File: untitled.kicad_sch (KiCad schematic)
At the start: 37 parts, among them J13 RaspPi_Conn, J15 UART_Bridge_TXRX, J16 Test_Conns, J3 USB_B_Micro, SW1 SW_Push, SW2 SW_Push, U3 ESP32-S3-WROOM-1

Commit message: after connor fixed footprints and billy started layout
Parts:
- C1, C11, C2: footprint CustomComponents:CAPC2012X95N_ -> LocalComponents:CAPC2012X95N_
- C8: footprint CustomComponents:CAPC1608X100N -> LocalComponents:CAPC1608X100N
- C9: footprint CustomComponents:CAPC1005X55N -> LocalComponents:CAPC1005X55N
- D11, D16: footprint CustomComponents:ESD5V0LBTP -> LocalComponents:ESD5V0LBTP
- J3: footprint CustomComponents:CONN_UB-MC5BR3-SDWP604-4S-TF_JST -> LocalComponents:CONN_UB-MC5BR3-SDWP604-4S-TF_JST
- R13, R21: footprint CustomComponents:RESC1005X40 -> LocalComponents:RESC1005X40
- R14: footprint CustomComponents:STA_RMCF0402_STP -> LocalComponents:STA_RMCF0402_STP
- R35: footprint CustomComponents:RESC2012X60N -> LocalComponents:RESC2012X60N
- SW1, SW2: footprint (none) -> LocalComponents:ESB335_PAN
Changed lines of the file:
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@@
 			)
 		)
-		(property "Footprint" "CustomComponents:CAPC2012X95N_"
+		(property "Footprint" "LocalComponents:CAPC2012X95N_"
 			(at 113.03 101.2952 0)
 			(effects
@@
 			)
 		)
-		(property "Footprint" "CustomComponents:CAPC2012X95N_"
+		(property "Footprint" "LocalComponents:CAPC2012X95N_"
 			(at 35.2552 44.45 0)
 			(effects
@@
 			)
 		)
-		(property "Footprint" "CustomComponents:CAPC1005X55N"
+		(property "Footprint" "LocalComponents:CAPC1005X55N"
 			(at 158.4452 40.64 0)
 			(effects
@@
 			)
 		)
-		(property "Footprint" "CustomComponents:ESD5V0LBTP"
+		(property "Footprint" "LocalComponents:ESD5V0LBTP"
 			(at 55.88 113.03 0)
 			(effects
@@
 			)
 		)
-		(property "Footprint" "CustomComponents:RESC1005X40"
+		(property "Footprint" "LocalComponents:RESC1005X40"
 			(at 28.702 77.47 90)
 			(effects
@@
 			)
 		)
-		(property "Footprint" "CustomComponents:RESC1005X40"
+		(property "Footprint" "LocalComponents:RESC1005X40"
 			(at 37.592 77.47 90)
 			(effects
@@
 			)
 		)
-		(property "Footprint" ""
+		(property "Footprint" "LocalComponents:ESB335_PAN"
 			(at 109.22 88.9 0)
 			(effects
@@
 			)
 		)
-		(property "Datasheet" "~"
+		(property "Datasheet" "https://www.digikey.com/en/products/detail/panasonic-electronic-components/ESB-33535A/3873298"
 			(at 109.22 88.9 0)
 			(effects
@@
 			)
 		)
-		(property "Footprint" "CustomComponents:STA_RMCF0402_STP"
+		(property "Footprint" "LocalComponents:STA_RMCF0402_STP"
 			(at 155.702 25.4 90)
 			(effects
@@
 			)
 		)
-		(property "Footprint" "CustomComponents:RESC2012X60N"
+		(property "Footprint" "LocalComponents:RESC2012X60N"
 			(at 14.732 115.57 90)
 			(effects
@@
 			)
 		)
-		(property "Footprint" ""
+		(property "Footprint" "LocalComponents:ESB335_PAN"
 			(at 109.22 125.73 0)
 			(effects
@@
 			)
 		)
-		(property "Datasheet" "~"
+		(property "Datasheet" "https://www.digikey.com/en/products/detail/panasonic-electronic-components/ESB-33535A/3873298"
 			(at 109.22 125.73 0)
 			(effects
@@
 			)
 		)
-		(property "Footprint" "CustomComponents:CONN_UB-MC5BR3-SDWP604-4S-TF_JST"
+		(property "Footprint" "LocalComponents:CONN_UB-MC5BR3-SDWP604-4S-TF_JST"
 			(at 22.86 102.87 0)
 			(effects
@@
 			)
 		)
-		(property "Footprint" "CustomComponents:CAPC2012X95N_"
+		(property "Footprint" "LocalComponents:CAPC2012X95N_"
 			(at 113.03 138.1252 0)
 			(effects
@@
 			)
 		)
-		(property "Footprint" "CustomComponents:CAPC1608X100N"
+		(property "Footprint" "LocalComponents:CAPC1608X100N"
 			(at 23.8252 44.45 0)
 			(effects
@@
 			)
 		)
-		(property "Footprint" "CustomComponents:ESD5V0LBTP"
+		(property "Footprint" "LocalComponents:ESD5V0LBTP"
 			(at 46.99 118.11 0)
 			(effects

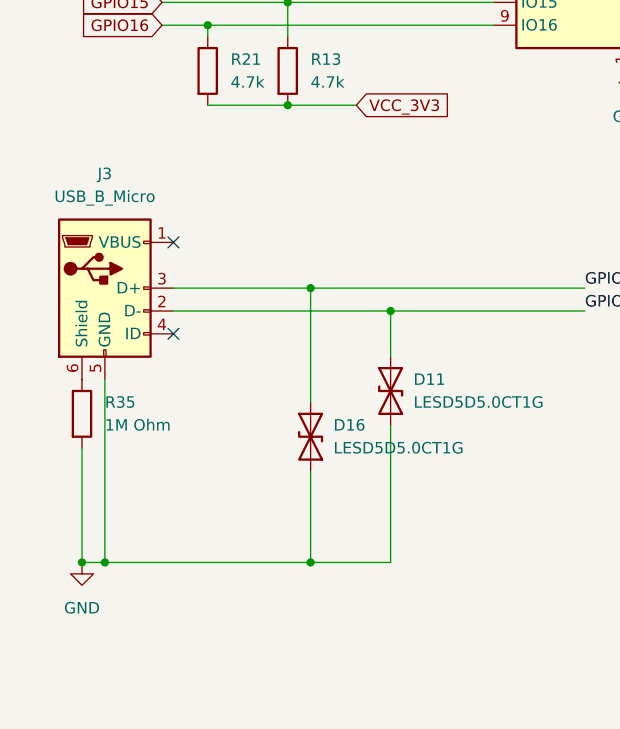
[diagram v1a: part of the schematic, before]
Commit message: pcb layout done, billy watching over us
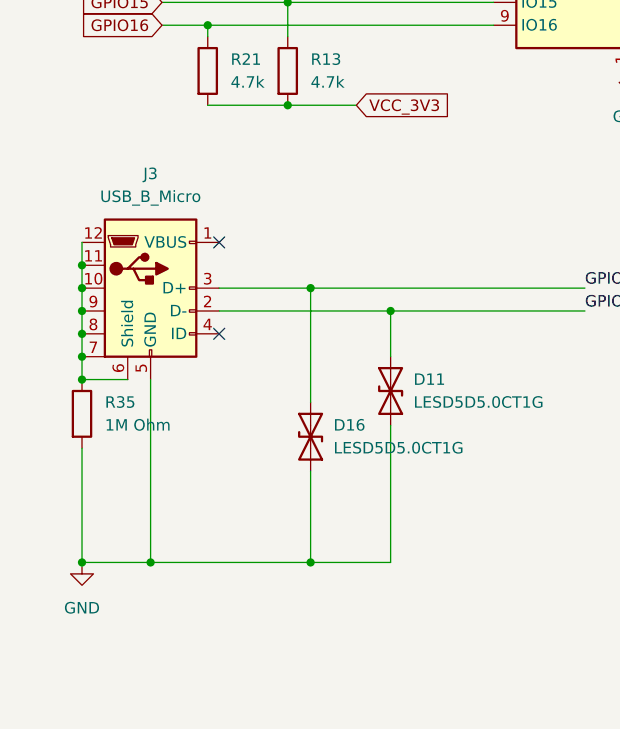
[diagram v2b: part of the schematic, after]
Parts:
- SW1, SW2: footprint LocalComponents:ESB335_PAN -> Button_Switch_THT:SW_PUSH-12mm
- TP1, TP2: footprint (none) -> TestPoint:TestPoint_Pad_D1.5mm
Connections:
- net at J3.6 (Shield), R35.1: now also J3.10, J3.11, J3.12, J3.7, J3.8, J3.9
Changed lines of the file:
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@@
 	)
 	(junction
+		(at 16.51 99.06)
+		(diameter 0)
+		(color 0 0 0 0)
+	)
+	(junction
+		(at 16.51 101.6)
+		(diameter 0)
+		(color 0 0 0 0)
+	)
+	(junction
 		(at 220.98 73.66)
 		(diameter 0)
@@
 	)
 	(junction
+		(at 16.51 106.68)
+		(diameter 0)
+		(color 0 0 0 0)
+	)
+	(junction
 		(at 165.1 120.65)
 		(diameter 0)
@@
 	)
 	(junction
-		(at 19.05 132.08)
+		(at 116.84 100.33)
 		(diameter 0)
 		(color 0 0 0 0)
 	)
 	(junction
-		(at 116.84 100.33)
+		(at 50.8 104.14)
 		(diameter 0)
 		(color 0 0 0 0)
 	)
 	(junction
-		(at 50.8 104.14)
+		(at 24.13 132.08)
 		(diameter 0)
 		(color 0 0 0 0)
@@
 	)
 	(junction
+		(at 16.51 109.22)
+		(diameter 0)
+		(color 0 0 0 0)
+	)
+	(junction
 		(at 127 25.4)
 		(diameter 0)
@@
 	)
 	(junction
+		(at 16.51 111.76)
+		(diameter 0)
+		(color 0 0 0 0)
+	)
+	(junction
 		(at 39.37 69.85)
 		(diameter 0)
@@
 	)
 	(junction
+		(at 16.51 104.14)
+		(diameter 0)
+		(color 0 0 0 0)
+	)
+	(junction
 		(at 226.06 86.36)
 		(diameter 0)
@@
 	)
 	(no_connect
-		(at 26.67 96.52)
+		(at 31.75 96.52)
 	)
 	(no_connect
@@
 	)
 	(no_connect
-		(at 26.67 106.68)
+		(at 31.75 106.68)
 	)
 	(no_connect
@@
 	(wire
 		(pts
+			(xy 16.51 99.06) (xy 16.51 101.6)
+		)
+		(stroke
+			(width 0)
+			(type default)
+		)
+	)
+	(wire
+		(pts
 			(xy 226.06 73.66) (xy 220.98 73.66)
 		)
@@
 	(wire
 		(pts
-			(xy 92.71 62.23) (xy 95.25 62.23)
+			(xy 24.13 132.08) (xy 41.91 132.08)
 		)
 		(stroke
@@
 	(wire
 		(pts
-			(xy 157.48 30.48) (xy 171.45 30.48)
+			(xy 92.71 62.23) (xy 95.25 62.23)
 		)
 		(stroke
@@
 	(wire
 		(pts
-			(xy 19.05 132.08) (xy 41.91 132.08)
+			(xy 157.48 30.48) (xy 171.45 30.48)
 		)
 		(stroke
@@
 	(wire
 		(pts
+			(xy 16.51 109.22) (xy 16.51 111.76)
+		)
+		(stroke
+			(width 0)
+			(type default)
+		)
+	)
+	(wire
+		(pts
 			(xy 238.76 41.91) (xy 260.35 41.91)
 		)
@@
 	(wire
 		(pts
+			(xy 16.51 101.6) (xy 16.51 104.14)
+		)
+		(stroke
+			(width 0)
+			(type default)
+		)
+	)
+	(wire
+		(pts
 			(xy 165.1 99.06) (xy 165.1 91.44)
 		)
@@
 	(wire
 		(pts
-			(xy 26.67 104.14) (xy 50.8 104.14)
+			(xy 31.75 104.14) (xy 50.8 104.14)
 		)
 		(stroke
@@
 	(wire
 		(pts
-			(xy 16.51 132.08) (xy 19.05 132.08)
+			(xy 16.51 132.08) (xy 24.13 132.08)
 		)
 		(stroke
@@
 	(wire
 		(pts
+			(xy 16.51 106.68) (xy 16.51 109.22)
+		)
+		(stroke
+			(width 0)
+			(type default)
+		)
+	)
+	(wire
+		(pts
 			(xy 157.48 19.05) (xy 157.48 21.59)
 		)
@@
 	(wire
 		(pts
-			(xy 26.67 101.6) (xy 41.91 101.6)
+			(xy 31.75 101.6) (xy 41.91 101.6)
 		)
 		(stroke
@@
 	(wire
 		(pts
+			(xy 21.59 111.76) (xy 16.51 111.76)
+		)
+		(stroke
+			(width 0)
+			(type default)
+		)
+	)
+	(wire
+		(pts
 			(xy 276.86 26.67) (xy 276.86 33.02)
 		)
@@
 	(wire
 		(pts
+			(xy 16.51 96.52) (xy 16.51 99.06)
+		)
+		(stroke
+			(width 0)
+			(type default)
+		)
+	)
+	(wire
+		(pts
 			(xy 22.86 44.45) (xy 22.86 46.99)
 		)
@@
 	(wire
 		(pts
+			(xy 16.51 104.14) (xy 16.51 106.68)
+		)
+		(stroke
+			(width 0)
+			(type default)
+		)
+	)
+	(wire
+		(pts
 			(xy 118.11 30.48) (xy 128.27 30.48)
 		)
@@
 	(wire
 		(pts
-			(xy 19.05 111.76) (xy 19.05 132.08)
+			(xy 24.13 111.76) (xy 24.13 132.08)
 		)
 		(stroke
@@
 			)
 		)
-		(property "Footprint" "LocalComponents:ESB335_PAN"
+		(property "Footprint" "Button_Switch_THT:SW_PUSH-12mm"
 			(at 109.22 88.9 0)
 			(effects
@@
 			)
 		)
-		(property "Footprint" "LocalComponents:ESB335_PAN"
+		(property "Footprint" "Button_Switch_THT:SW_PUSH-12mm"
 			(at 109.22 125.73 0)
 			(effects
@@
 	(symbol
 		(lib_id "Connector:USB_B_Micro")
-		(at 19.05 101.6 0)
+		(at 24.13 101.6 0)
 		(unit 1)
 		(exclude_from_sim no)
@@
 		(fields_autoplaced yes)
 		(property "Reference" "J3"
-			(at 19.05 88.9 0)
+			(at 24.13 88.9 0)
 			(effects
 				(font
@@
 		)
 		(property "Value" "USB_B_Micro"
-			(at 19.05 91.44 0)
+			(at 24.13 91.44 0)
 			(effects
 				(font
@@
 		)
 		(property "Footprint" "LocalComponents:CONN_UB-MC5BR3-SDWP604-4S-TF_JST"
-			(at 22.86 102.87 0)
+			(at 27.94 102.87 0)
 			(effects
 				(font
@@
 		)
 		(property "Datasheet" "https://www.jst-mfg.com/product/pdf/eng/eUB-micro-USB1.pdf"
-			(at 22.86 102.87 0)
+			(at 27.94 102.87 0)
 			(effects
 				(font
@@
 		)
 		(property "Description" "USB Micro Type B connector"
-			(at 19.05 101.6 0)
+			(at 24.13 101.6 0)
 			(effects
 				(font
@@
 		(pin "1"
 		)
+		(pin "12"
+		)
+		(pin "11"
+		)
+		(pin "10"
+		)
+		(pin "9"
+		)
+		(pin "8"
+		)
+		(pin "7"
+		)
 		(instances
 			(project "PCB_draft1"
@@
 			)
 		)
-		(property "Footprint" ""
+		(property "Footprint" "TestPoint:TestPoint_Pad_D1.5mm"
 			(at 121.92 128.27 0)
 			(effects
@@
 			)
 		)
-		(property "Footprint" ""
+		(property "Footprint" "TestPoint:TestPoint_Pad_D1.5mm"
 			(at 121.92 91.44 0)
 			(effects

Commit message: pcb draft 2 from billy
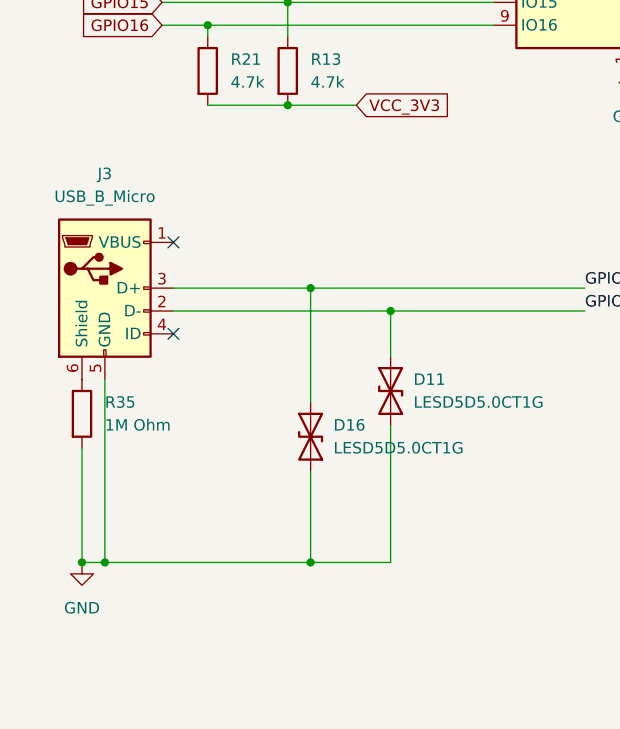
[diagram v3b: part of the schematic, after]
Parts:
- R13, R21: footprint LocalComponents:RESC1005X40 -> Resistor_SMD:R_0805_2012Metric_Pad1.20x1.40mm_HandSolder
- R14: footprint LocalComponents:STA_RMCF0402_STP -> Resistor_SMD:R_0805_2012Metric_Pad1.20x1.40mm_HandSolder
- R35: footprint LocalComponents:RESC2012X60N -> Resistor_SMD:R_0805_2012Metric_Pad1.20x1.40mm_HandSolder
- SW1, SW2: footprint Button_Switch_THT:SW_PUSH-12mm -> LocalComponents:ESB335_PAN
- TP1, TP2: footprint TestPoint:TestPoint_Pad_D1.5mm -> TestPoint_Pad_D1.0mm
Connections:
- new net: J3.6 (Shield), R35.1
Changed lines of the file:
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@@
 	)
 	(junction
-		(at 16.51 99.06)
-		(diameter 0)
-		(color 0 0 0 0)
-	)
-	(junction
-		(at 16.51 101.6)
-		(diameter 0)
-		(color 0 0 0 0)
-	)
-	(junction
 		(at 220.98 73.66)
 		(diameter 0)
@@
 	)
 	(junction
-		(at 16.51 106.68)
-		(diameter 0)
-		(color 0 0 0 0)
-	)
-	(junction
 		(at 165.1 120.65)
 		(diameter 0)
@@
 	)
 	(junction
-		(at 116.84 100.33)
+		(at 19.05 132.08)
 		(diameter 0)
 		(color 0 0 0 0)
 	)
 	(junction
-		(at 50.8 104.14)
+		(at 116.84 100.33)
 		(diameter 0)
 		(color 0 0 0 0)
 	)
 	(junction
-		(at 24.13 132.08)
+		(at 50.8 104.14)
 		(diameter 0)
 		(color 0 0 0 0)
@@
 	)
 	(junction
-		(at 16.51 109.22)
-		(diameter 0)
-		(color 0 0 0 0)
-	)
-	(junction
 		(at 127 25.4)
 		(diameter 0)
@@
 	)
 	(junction
-		(at 16.51 111.76)
-		(diameter 0)
-		(color 0 0 0 0)
-	)
-	(junction
 		(at 39.37 69.85)
 		(diameter 0)
@@
 	)
 	(junction
-		(at 16.51 104.14)
-		(diameter 0)
-		(color 0 0 0 0)
-	)
-	(junction
 		(at 226.06 86.36)
 		(diameter 0)
@@
 	)
 	(no_connect
-		(at 31.75 96.52)
+		(at 26.67 96.52)
 	)
 	(no_connect
@@
 	)
 	(no_connect
-		(at 31.75 106.68)
+		(at 26.67 106.68)
 	)
 	(no_connect
@@
 	(wire
 		(pts
-			(xy 16.51 99.06) (xy 16.51 101.6)
-		)
-		(stroke
-			(width 0)
-			(type default)
-		)
-	)
-	(wire
-		(pts
 			(xy 226.06 73.66) (xy 220.98 73.66)
 		)
@@
 	(wire
 		(pts
-			(xy 24.13 132.08) (xy 41.91 132.08)
+			(xy 92.71 62.23) (xy 95.25 62.23)
 		)
 		(stroke
@@
 	(wire
 		(pts
-			(xy 92.71 62.23) (xy 95.25 62.23)
+			(xy 157.48 30.48) (xy 171.45 30.48)
 		)
 		(stroke
@@
 	(wire
 		(pts
-			(xy 157.48 30.48) (xy 171.45 30.48)
+			(xy 19.05 132.08) (xy 41.91 132.08)
 		)
 		(stroke
@@
 	(wire
 		(pts
-			(xy 16.51 109.22) (xy 16.51 111.76)
-		)
-		(stroke
-			(width 0)
-			(type default)
-		)
-	)
-	(wire
-		(pts
 			(xy 238.76 41.91) (xy 260.35 41.91)
 		)
@@
 	(wire
 		(pts
-			(xy 16.51 101.6) (xy 16.51 104.14)
-		)
-		(stroke
-			(width 0)
-			(type default)
-		)
-	)
-	(wire
-		(pts
 			(xy 165.1 99.06) (xy 165.1 91.44)
 		)
@@
 	(wire
 		(pts
-			(xy 31.75 104.14) (xy 50.8 104.14)
+			(xy 26.67 104.14) (xy 50.8 104.14)
 		)
 		(stroke
@@
 	(wire
 		(pts
-			(xy 16.51 132.08) (xy 24.13 132.08)
+			(xy 16.51 132.08) (xy 19.05 132.08)
 		)
 		(stroke
@@
 	(wire
 		(pts
-			(xy 16.51 106.68) (xy 16.51 109.22)
-		)
-		(stroke
-			(width 0)
-			(type default)
-		)
-	)
-	(wire
-		(pts
 			(xy 157.48 19.05) (xy 157.48 21.59)
 		)
@@
 	(wire
 		(pts
-			(xy 31.75 101.6) (xy 41.91 101.6)
+			(xy 26.67 101.6) (xy 41.91 101.6)
 		)
 		(stroke
@@
 	(wire
 		(pts
-			(xy 21.59 111.76) (xy 16.51 111.76)
-		)
-		(stroke
-			(width 0)
-			(type default)
-		)
-	)
-	(wire
-		(pts
 			(xy 276.86 26.67) (xy 276.86 33.02)
 		)
@@
 	(wire
 		(pts
-			(xy 16.51 96.52) (xy 16.51 99.06)
-		)
-		(stroke
-			(width 0)
-			(type default)
-		)
-	)
-	(wire
-		(pts
 			(xy 22.86 44.45) (xy 22.86 46.99)
 		)
@@
 	(wire
 		(pts
-			(xy 16.51 104.14) (xy 16.51 106.68)
-		)
-		(stroke
-			(width 0)
-			(type default)
-		)
-	)
-	(wire
-		(pts
 			(xy 118.11 30.48) (xy 128.27 30.48)
 		)
@@
 	(wire
 		(pts
-			(xy 24.13 111.76) (xy 24.13 132.08)
+			(xy 19.05 111.76) (xy 19.05 132.08)
 		)
 		(stroke
@@
 			)
 		)
-		(property "Footprint" "LocalComponents:RESC1005X40"
+		(property "Footprint" "Resistor_SMD:R_0805_2012Metric_Pad1.20x1.40mm_HandSolder"
 			(at 28.702 77.47 90)
 			(effects
@@
 			)
 		)
-		(property "Footprint" "LocalComponents:RESC1005X40"
+		(property "Footprint" "Resistor_SMD:R_0805_2012Metric_Pad1.20x1.40mm_HandSolder"
 			(at 37.592 77.47 90)
 			(effects
@@
 			)
 		)
-		(property "Footprint" "Button_Switch_THT:SW_PUSH-12mm"
+		(property "Footprint" "LocalComponents:ESB335_PAN"
 			(at 109.22 88.9 0)
 			(effects
@@
 			)
 		)
-		(property "Footprint" "LocalComponents:STA_RMCF0402_STP"
+		(property "Footprint" "Resistor_SMD:R_0805_2012Metric_Pad1.20x1.40mm_HandSolder"
 			(at 155.702 25.4 90)
 			(effects
@@
 			)
 		)
-		(property "Footprint" "LocalComponents:RESC2012X60N"
+		(property "Footprint" "Resistor_SMD:R_0805_2012Metric_Pad1.20x1.40mm_HandSolder"
 			(at 14.732 115.57 90)
 			(effects
@@
 			)
 		)
-		(property "Footprint" "Button_Switch_THT:SW_PUSH-12mm"
+		(property "Footprint" "LocalComponents:ESB335_PAN"
 			(at 109.22 125.73 0)
 			(effects
@@
 	(symbol
 		(lib_id "Connector:USB_B_Micro")
-		(at 24.13 101.6 0)
+		(at 19.05 101.6 0)
 		(unit 1)
 		(exclude_from_sim no)
@@
 		(fields_autoplaced yes)
 		(property "Reference" "J3"
-			(at 24.13 88.9 0)
+			(at 19.05 88.9 0)
 			(effects
 				(font
@@
 		)
 		(property "Value" "USB_B_Micro"
-			(at 24.13 91.44 0)
+			(at 19.05 91.44 0)
 			(effects
 				(font
@@
 		)
 		(property "Footprint" "LocalComponents:CONN_UB-MC5BR3-SDWP604-4S-TF_JST"
-			(at 27.94 102.87 0)
+			(at 22.86 102.87 0)
 			(effects
 				(font
@@
 		)
 		(property "Datasheet" "https://www.jst-mfg.com/product/pdf/eng/eUB-micro-USB1.pdf"
-			(at 27.94 102.87 0)
+			(at 22.86 102.87 0)
 			(effects
 				(font
@@
 		)
 		(property "Description" "USB Micro Type B connector"
-			(at 24.13 101.6 0)
+			(at 19.05 101.6 0)
 			(effects
 				(font
@@
 		(pin "1"
 		)
-		(pin "12"
-		)
-		(pin "11"
-		)
-		(pin "10"
-		)
-		(pin "9"
-		)
-		(pin "8"
-		)
-		(pin "7"
-		)
 		(instances
 			(project "PCB_draft1"
@@
 			)
 		)
-		(property "Footprint" "TestPoint:TestPoint_Pad_D1.5mm"
+		(property "Footprint" "TestPoint_Pad_D1.0mm"
 			(at 121.92 128.27 0)
 			(effects
@@
 			)
 		)
-		(property "Footprint" "TestPoint:TestPoint_Pad_D1.5mm"
+		(property "Footprint" "TestPoint_Pad_D1.0mm"
 			(at 121.92 91.44 0)
 			(effects
